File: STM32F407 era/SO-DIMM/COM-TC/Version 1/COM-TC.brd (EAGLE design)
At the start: 127 x 165.1 mm, 168 parts, among them J1 CON1, J2 CON1, J3 SO-DIMM-CPU, J4 FTDI_DEVICE, Q4 PMV20XNE, U1 IRF9332PBF, U10 SN65HVD232D, U11 MAX9926, U12 MCP6004-E/SL, U13 MCP6004-E/SL, U14 MCP6004-E/SL, U2 5V, U3 TPS54331D, U4 3,3V, U5 MAX9926, U6 MCP6004-E/SL, U7 LoPy, U8 GTL2000, X1 057-014-1

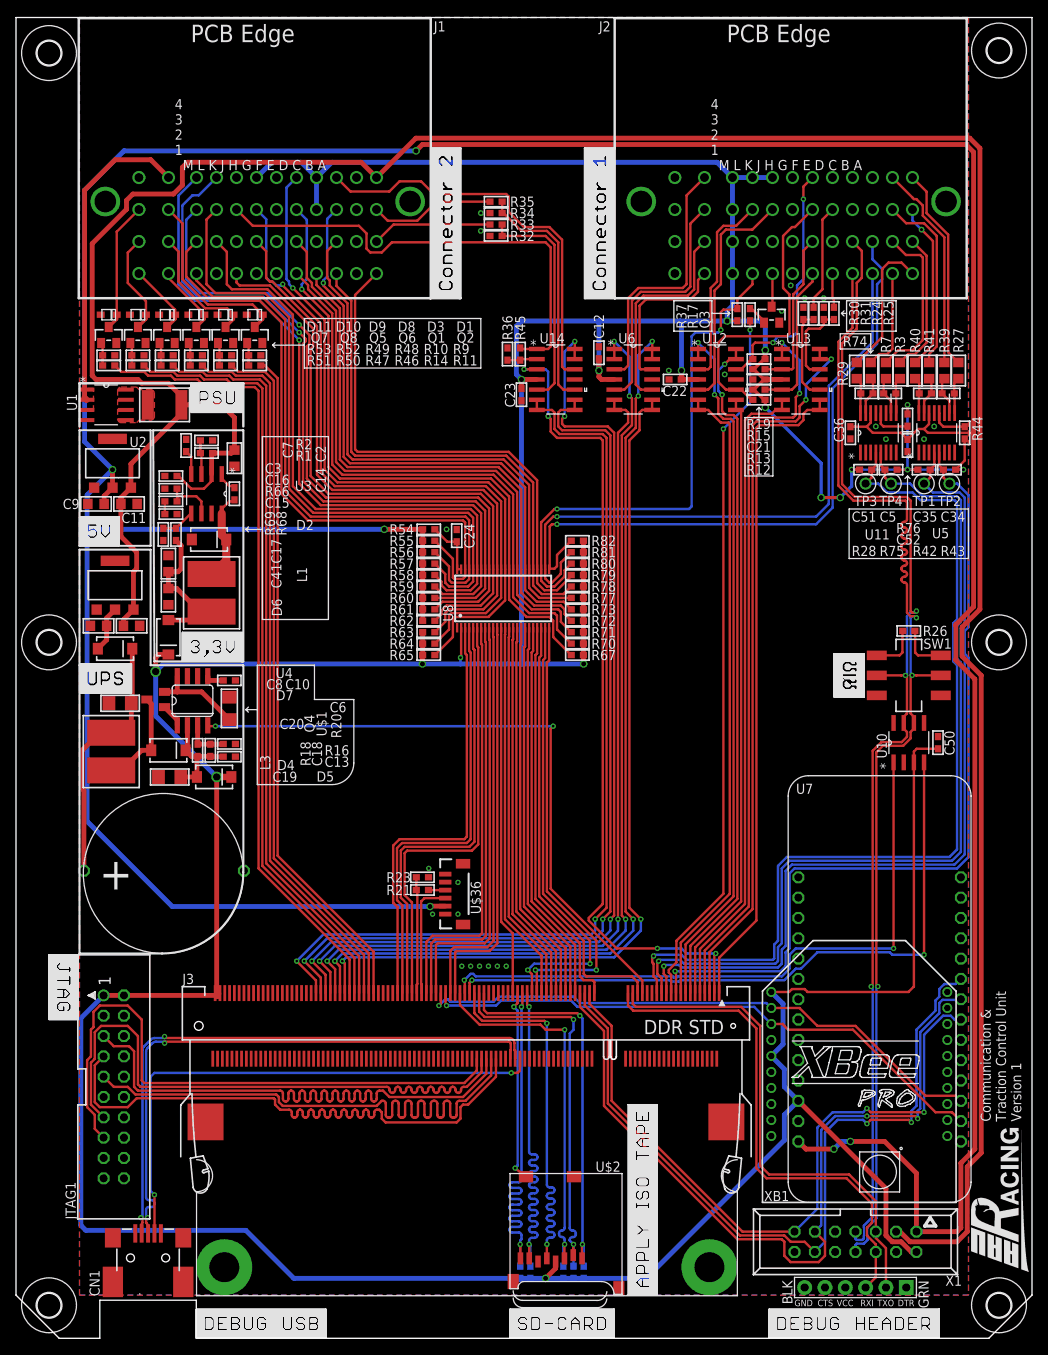
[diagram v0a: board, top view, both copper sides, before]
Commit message: All board V1-RC1 done
all boards ready for inspection
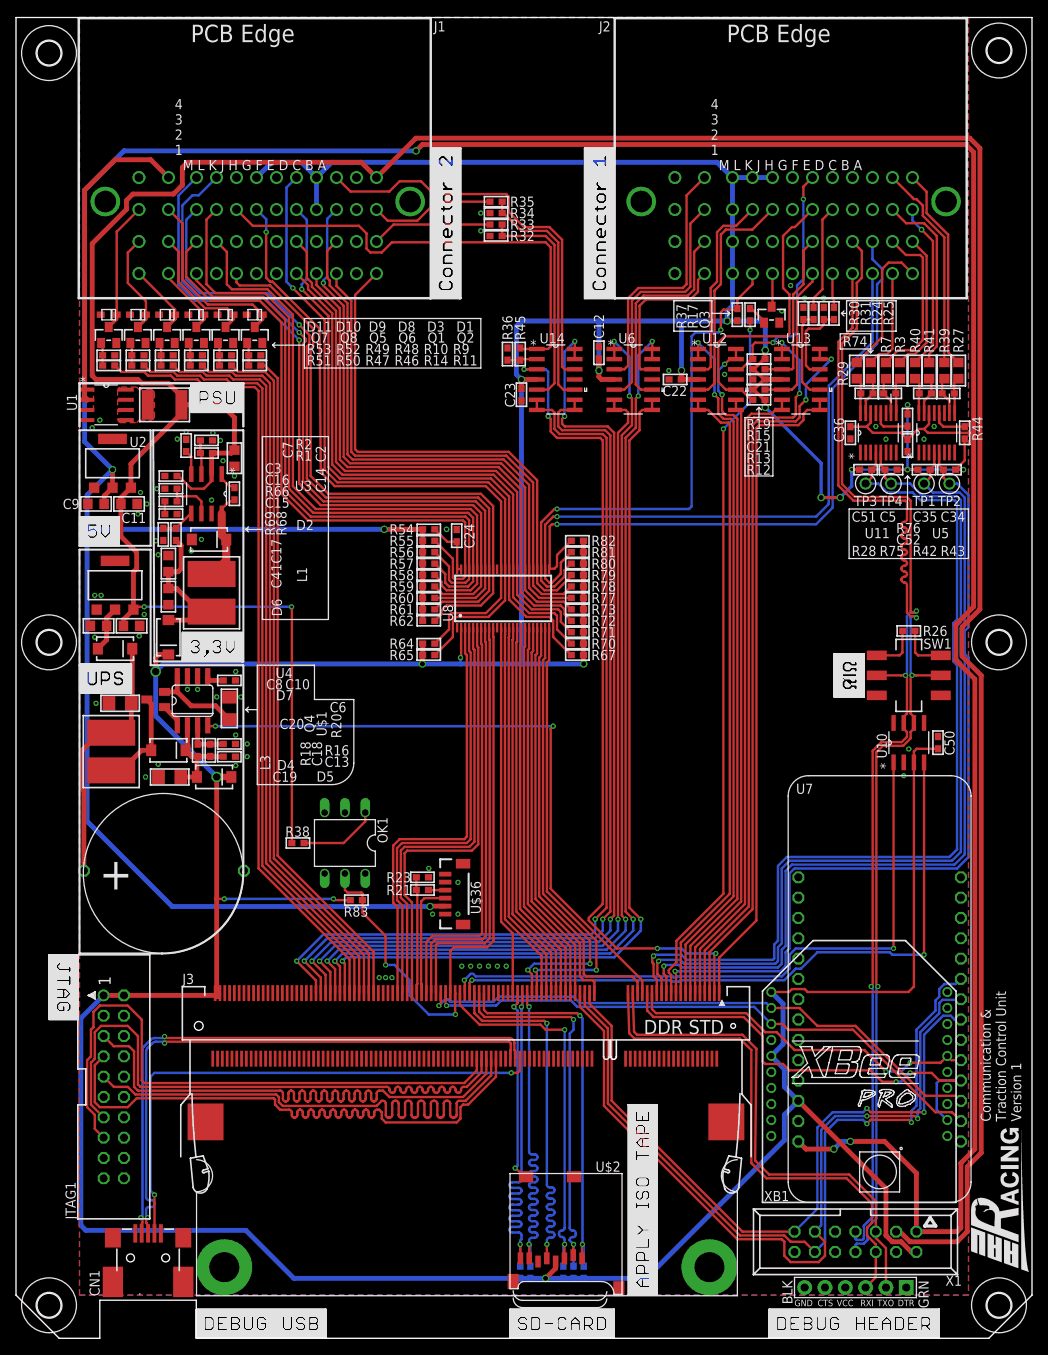
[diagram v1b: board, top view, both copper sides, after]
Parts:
- removed R63: 220, microbuilder:_0603
- added OK1: 4N33, optocoupler:DIL06
- added R38: 560, microbuilder:_0603
- added R83: 500, microbuilder:_0603
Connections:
- removed net AUX1: J1.G2, R63.2, U8.38
- removed net AUX1L: J3.99, U8.11
- new net CTS: J3.31, U7.23, XB1.12
- new net N$22: OK1.1, R38.2
- new net PWR_OUT: J3.99, OK1.5, R83.2
- new net RTS: J3.29, U7.24, XB1.16
- net 12V: now also R38.1
- net 3.3V: now also R83.1; no longer R63.1
- net GND: now also OK1.2, OK1.4
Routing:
- net AUX1: track 78.3 -> 0.00 mm
- net CTS: track 0.00 -> 56.1 mm, vias 0 -> 2
- net AUX1L: track 50.3 -> 0.00 mm
- net 12V: track 353.7 -> 403.2 mm, vias 0 -> 2
- net RTS: track 0.00 -> 44.9 mm, vias 0 -> 2
- net PWR_OUT: track 0.00 -> 29.7 mm, vias 0 -> 2
- net 3.3V: track 628.9 -> 644.2 mm, vias 18 -> 20
- net N$22: track 0.00 -> 9.88 mm
- net AUX2: track 84.8 -> 84.1 mm
